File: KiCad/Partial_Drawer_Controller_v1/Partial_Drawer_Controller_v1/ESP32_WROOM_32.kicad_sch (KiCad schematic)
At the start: 42 parts, among them Q1 SS8050, Q2 2N7002T-7-F, Q3 2N7002T-7-F, Q5 SS8050, U6 CP2102N-Axx-xQFN28, U7 ESP32-WROOM-32E-N8, X1 USB-Micro

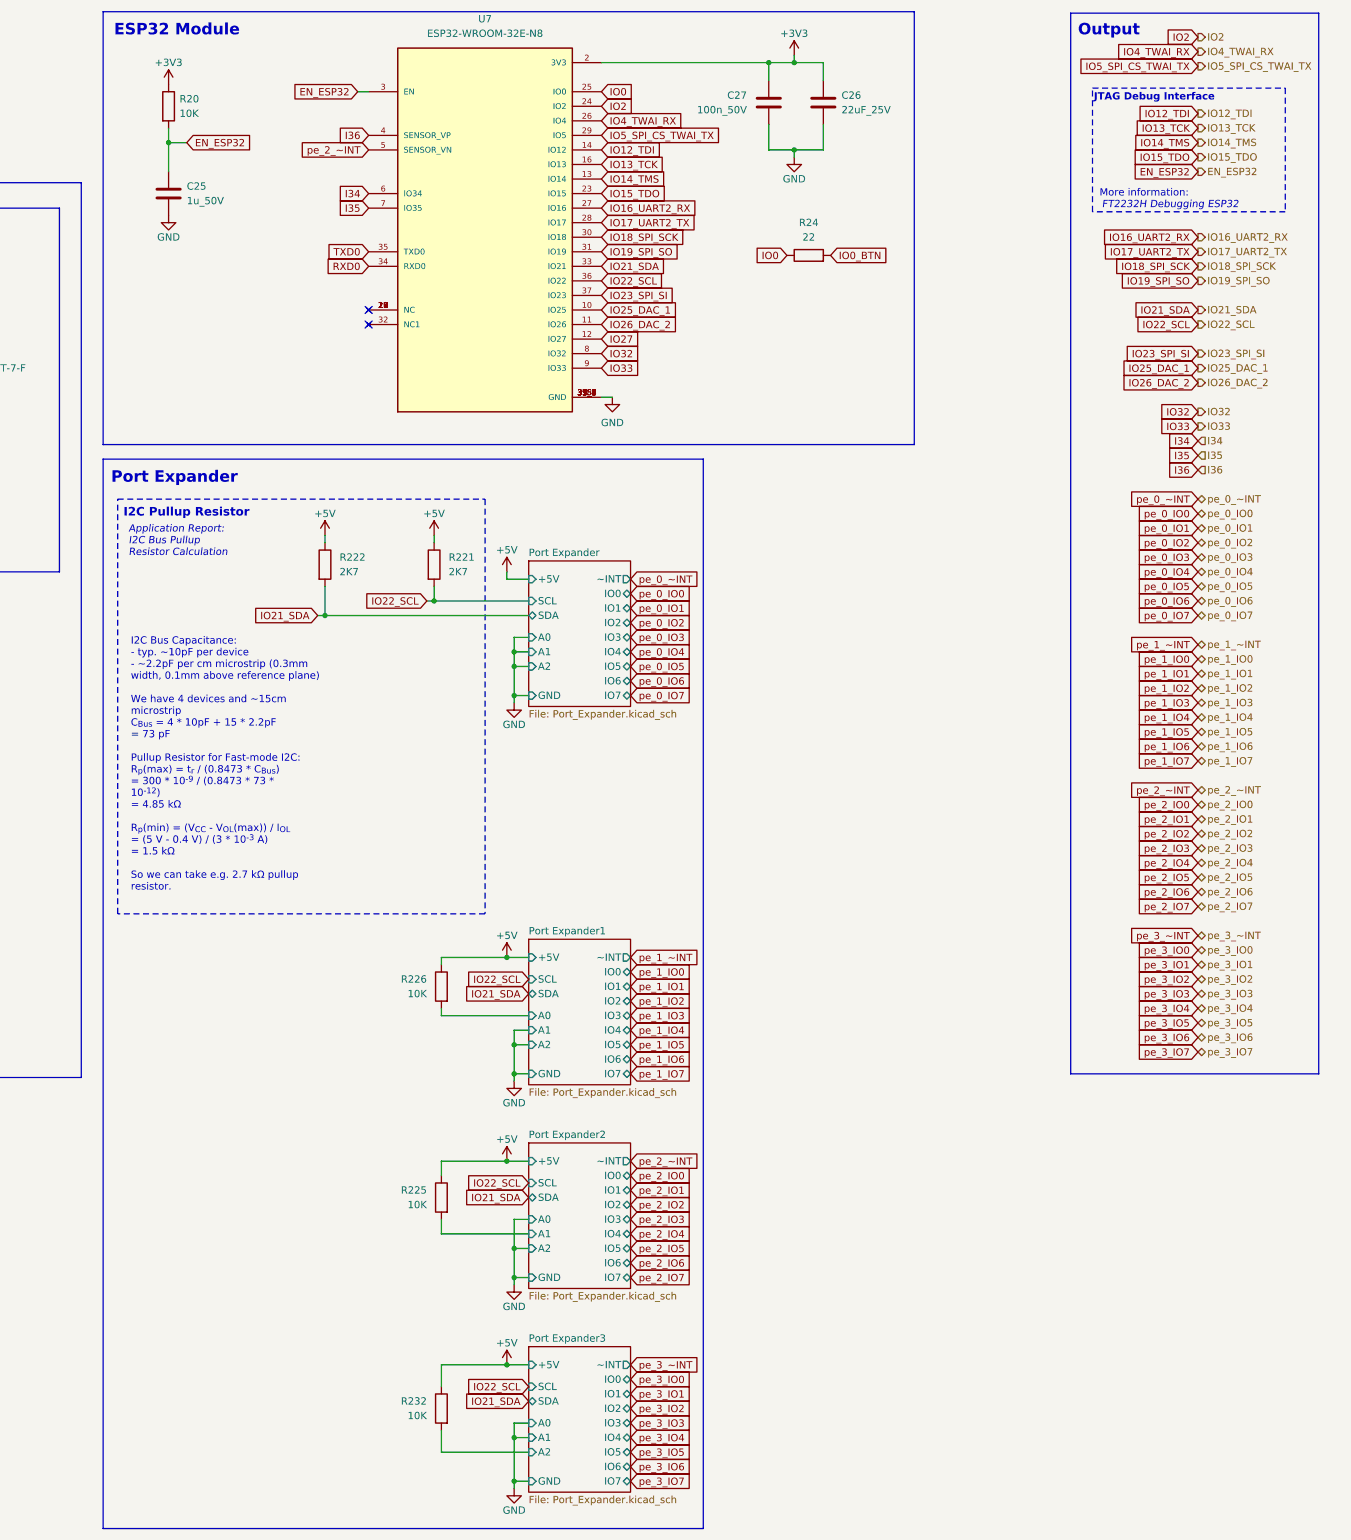
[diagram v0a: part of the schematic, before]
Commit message: feat: finishing first draft for `partial_drawer_controller_v1` schematic
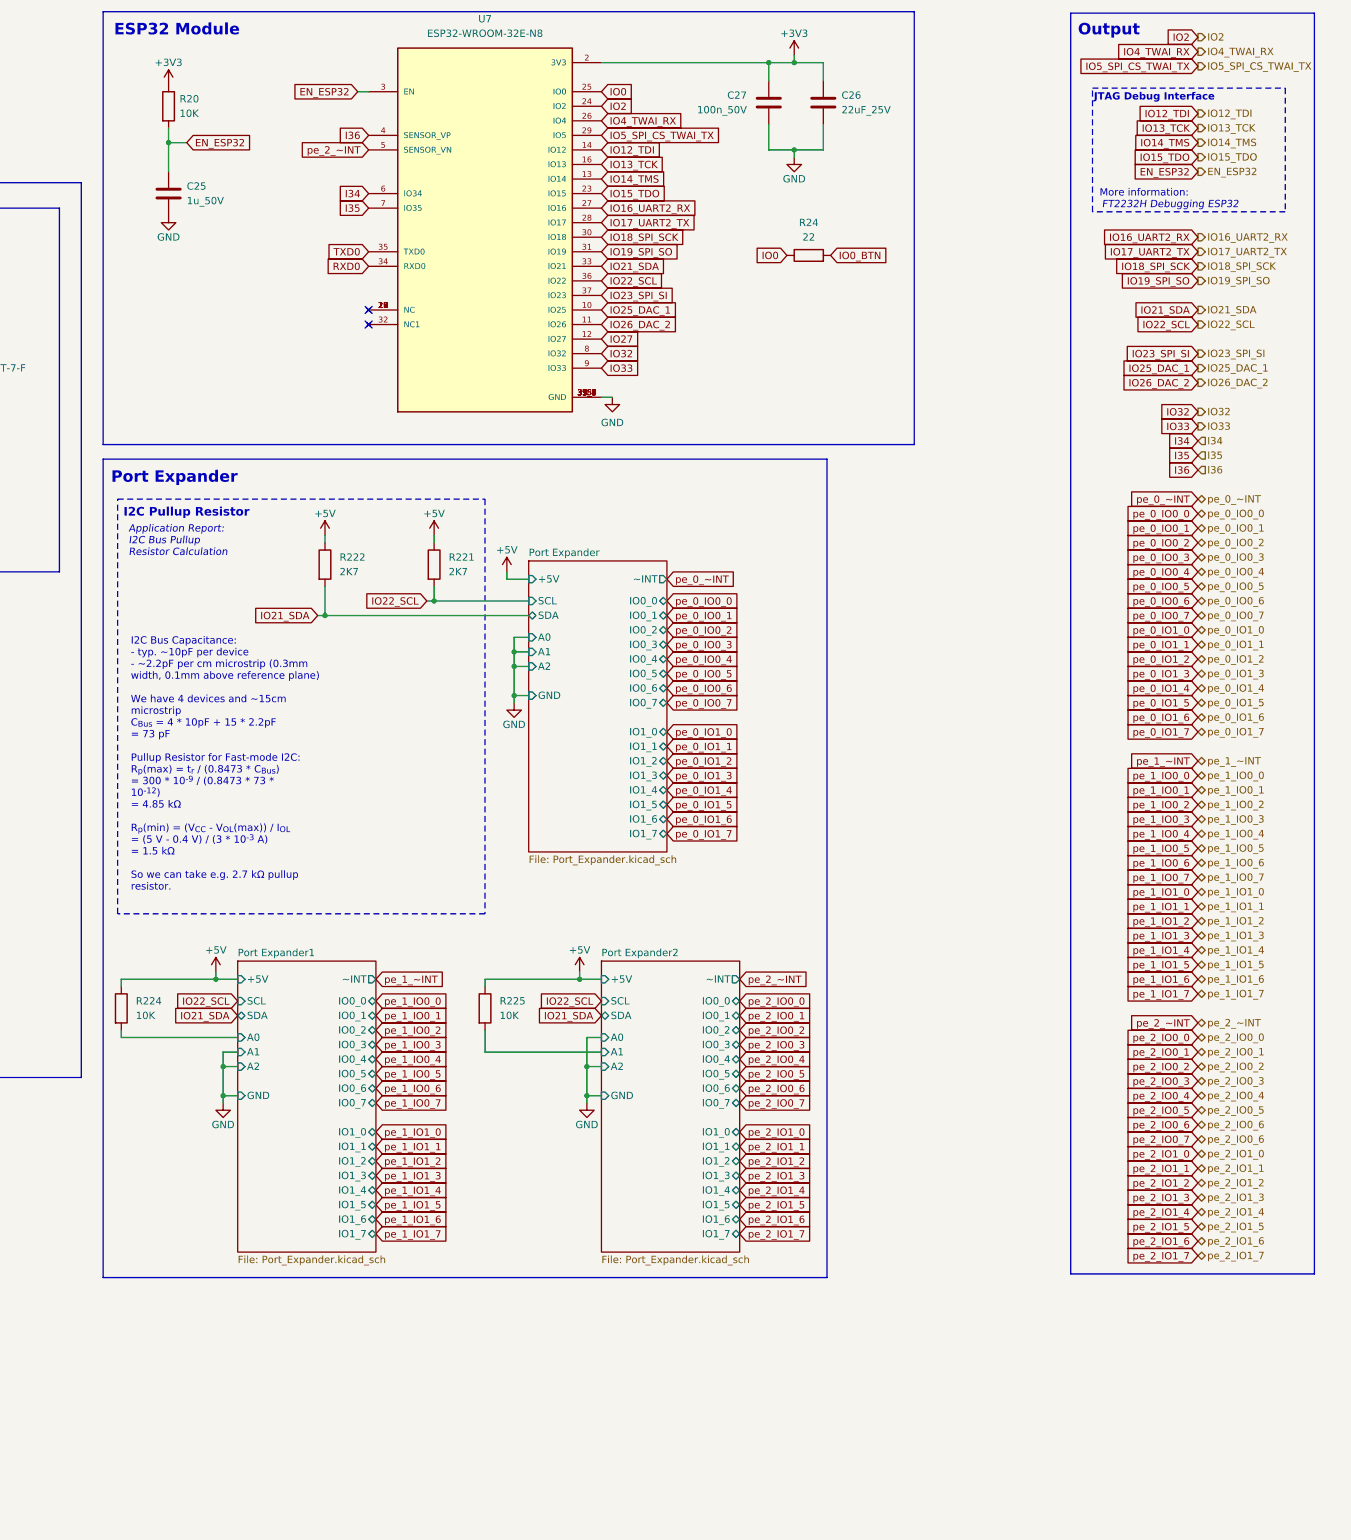
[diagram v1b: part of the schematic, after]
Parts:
- removed R226, R232: 10K, Resistor_SMD:R_0402_1005Metric, symbol _R_0402:10K
- added R224: 10K, Resistor_SMD:R_0402_1005Metric, symbol _R_0402:10K
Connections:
- net +5V: now also R224.1
- net Port Expander1/A0: now also R224.2
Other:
- removed sheet Port Expander3
- sheet Port Expander ports: added IO0_0, IO0_1, IO0_2, IO0_3, IO0_4, IO0_5, IO0_6, IO0_7, IO1_0, IO1_1, IO1_2, IO1_3, IO1_4, IO1_5, IO1_6, IO1_7; removed IO0, IO1, IO2, IO3, IO4, IO5, IO6, IO7
- sheet Port Expander1 ports: added IO0_0, IO0_1, IO0_2, IO0_3, IO0_4, IO0_5, IO0_6, IO0_7, IO1_0, IO1_1, IO1_2, IO1_3, IO1_4, IO1_5, IO1_6, IO1_7; removed IO0, IO1, IO2, IO3, IO4, IO5, IO6, IO7
- sheet Port Expander2 ports: added IO0_0, IO0_1, IO0_2, IO0_3, IO0_4, IO0_5, IO0_6, IO0_7, IO1_0, IO1_1, IO1_2, IO1_3, IO1_4, IO1_5, IO1_6, IO1_7; removed IO0, IO1, IO2, IO3, IO4, IO5, IO6, IO7
